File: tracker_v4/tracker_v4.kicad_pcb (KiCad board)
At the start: 4 copper layers, 63.2 x 26 mm, 66 parts, among them J1 USB_C_Receptacle_USB2.0_16P, Q1 DMG9926UDM-7, U1 ESP32-C6-MINI-1-N4, U2 LIS3DH, U3 DW01A, U4 INA226AIDGSR, U5 TPS63020, U6 USBLC6-2SC6, U7 TPS3899DL01DSER, U8 BQ24072RGT

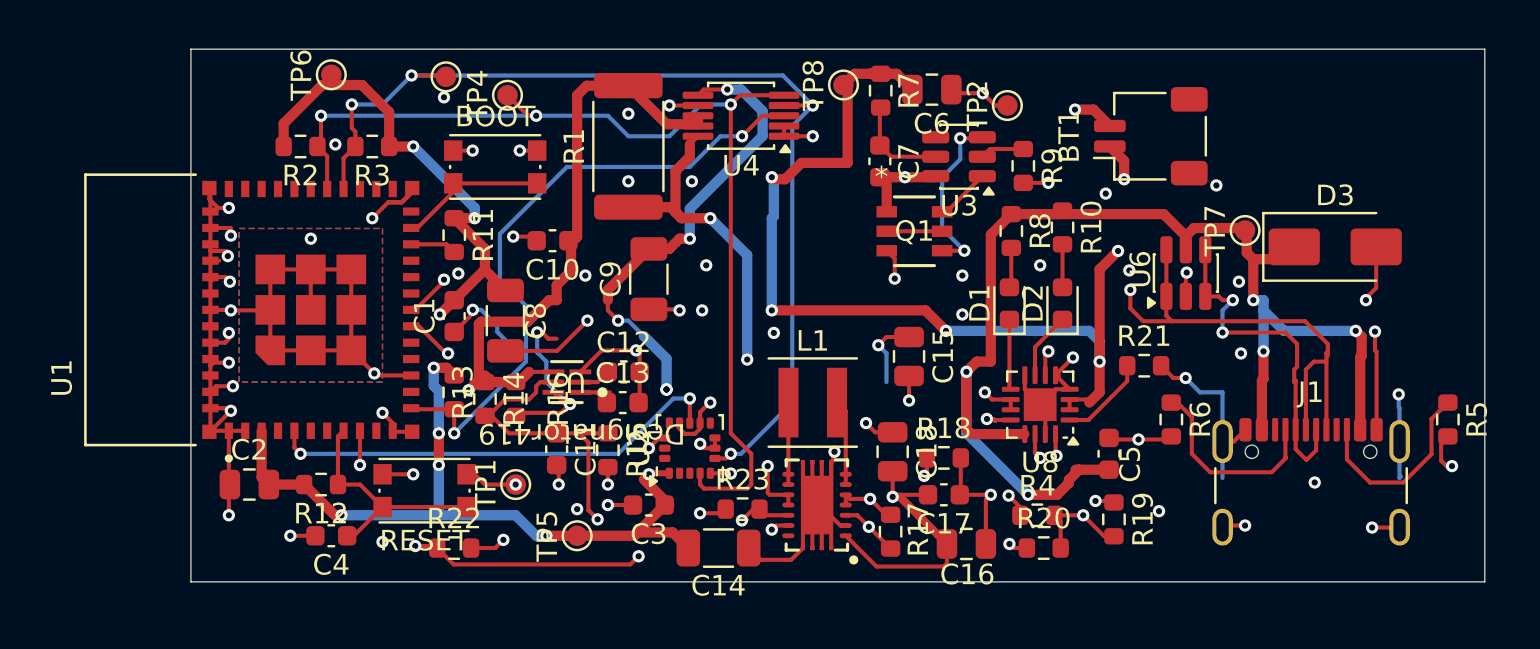
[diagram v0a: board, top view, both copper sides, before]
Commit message: b
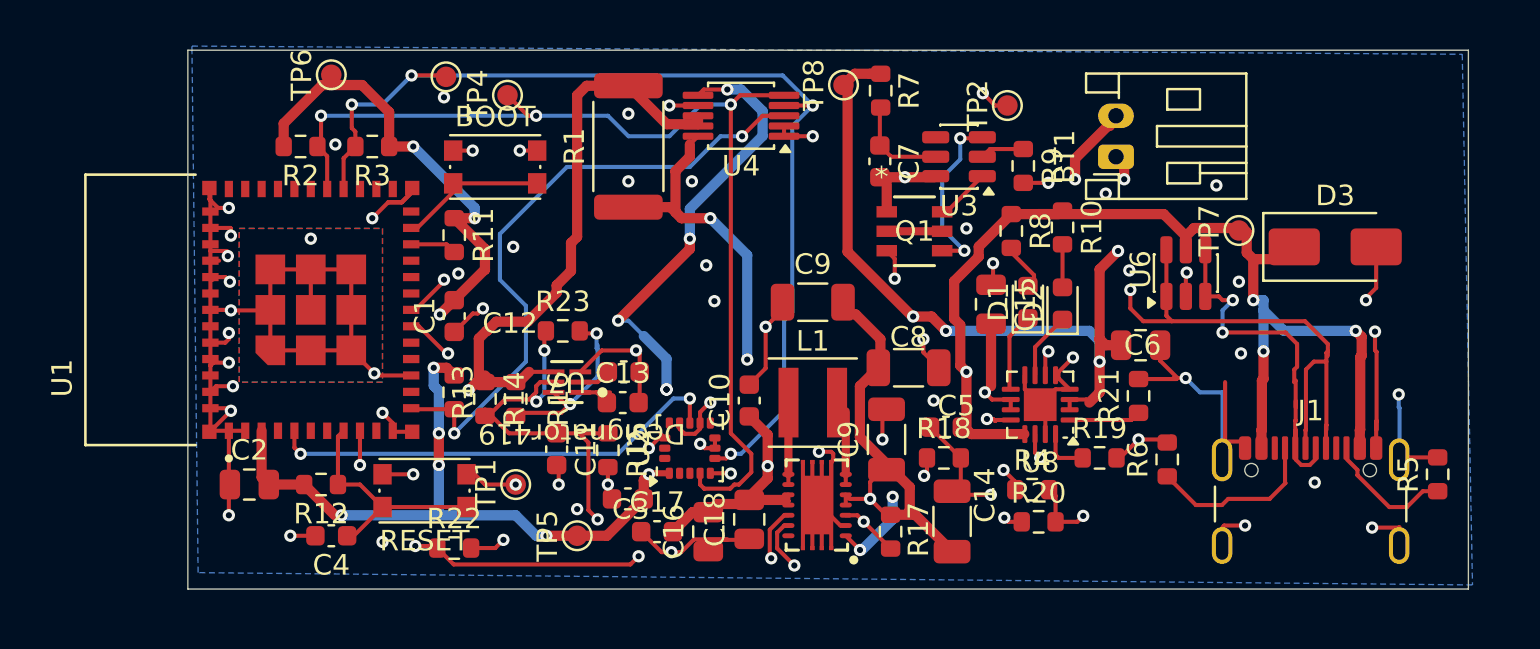
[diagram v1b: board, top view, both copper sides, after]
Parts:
- removed the C9 at (129.5, 109.0)
- added C9: 22u, Capacitor_SMD:C_1206_3216Metric, F.Cu at (141.1, 116.8)
- added C9: 22u, Capacitor_SMD:C_1206_3216Metric, F.Cu at (137.5, 110.1)
- BT1: footprint Connector_JST:JST_SH_SM02B-SRSS-TB_1x02-1MP_P1.00mm_Horizontal -> Connector_JST:JST_PH_S2B-PH-K_1x02_P2.00mm_Horizontal
- R7: value 500 -> 499
- moved C8 19.8 mm to (142.2, 113.3), turned to 0 degrees
- moved C6 16.1 mm to (153.5, 112.2)
- moved C17 14.1 mm to (129.9, 121.3), turned to 0 degrees
- moved C16 12.6 mm to (132.4, 121.3), turned to 90 degrees
- moved C10 12.4 mm to (134.4, 114.9), turned to 90 degrees
- moved R23 12.4 mm to (125.3, 111.5)
- moved C14 11.5 mm to (144.3, 120.8), turned to -90 degrees
- moved C5 8.07 mm to (144.0, 116.2), turned to 180 degrees
- moved C18 7.74 mm to (134.4, 120.7), turned to 90 degrees
- moved C15 4.74 mm to (146.2, 110.2)
- moved R19 3.08 mm to (151.5, 117.7), turned to 0 degrees
- moved R5 2.72 mm to (168.0, 118.5), turned to 90 degrees
- moved BT1 1.97 mm to (152.3, 103.0)
- moved R6 1.96 mm to (154.8, 117.8), turned to 90 degrees
- moved R21 1.50 mm to (153.4, 114.7), turned to 90 degrees
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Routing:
- net BAT+: track 51.4 -> 40.4 mm, vias 6 -> 5
- net 3v3: track 111.9 -> 122.7 mm
- net USB_VBUS: track 68.9 -> 58.9 mm, vias 6 -> 5
- net Net-(J1-CC2): track 9.47 -> 5.87 mm
- net BUCK_SYNC: track 26.1 -> 28.8 mm
- net Net-(U8-ISET): track 5.00 -> 2.40 mm, vias 2 -> 0
- net UVLO_SENSE: track 21.7 -> 19.3 mm, vias 2 -> 3
- net POWER_OUT: track 32.1 -> 34.4 mm
- net /Charging_and_Battery/BAT-: track 19.4 -> 17.4 mm
- net USB_DP: track 59.3 -> 61.4 mm
- net BUCK_EN: track 26.8 -> 28.3 mm
- net Net-(U8-ILIM): track 6.85 -> 5.52 mm
- net Net-(J1-CC1): track 9.74 -> 8.51 mm
- net SHUNT_OUTPUT: track 70.6 -> 69.5 mm, vias 3 -> 4
- net GND: track 165.4 -> 166.4 mm, vias 72 -> 66
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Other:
- board size 63.2 x 26 mm -> 62.5 x 26.3 mm
